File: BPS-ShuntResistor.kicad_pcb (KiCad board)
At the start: 2 copper layers, 37.6 x 32.5 mm, 9 parts, among them J1 Amp_Conn, J2 Conn_01x01_Female, J3 Conn_01x01_Female

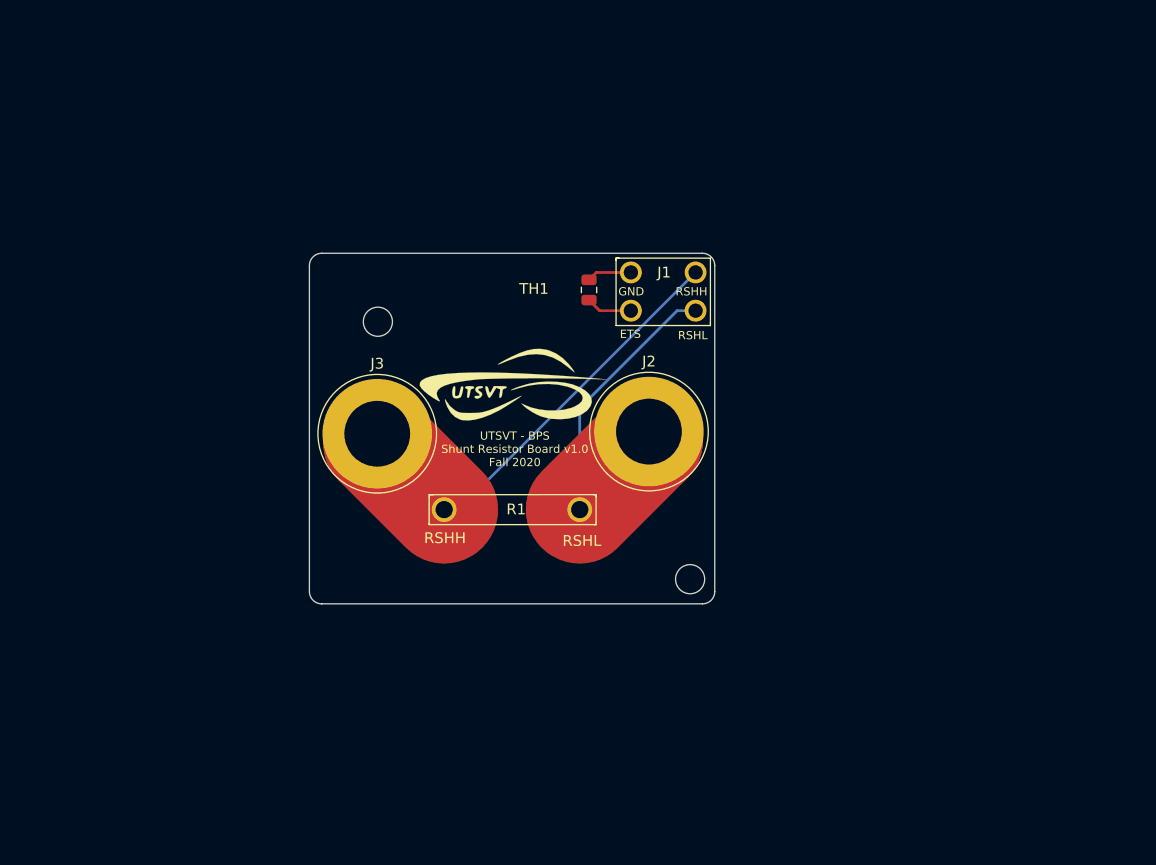
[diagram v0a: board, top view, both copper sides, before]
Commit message: a
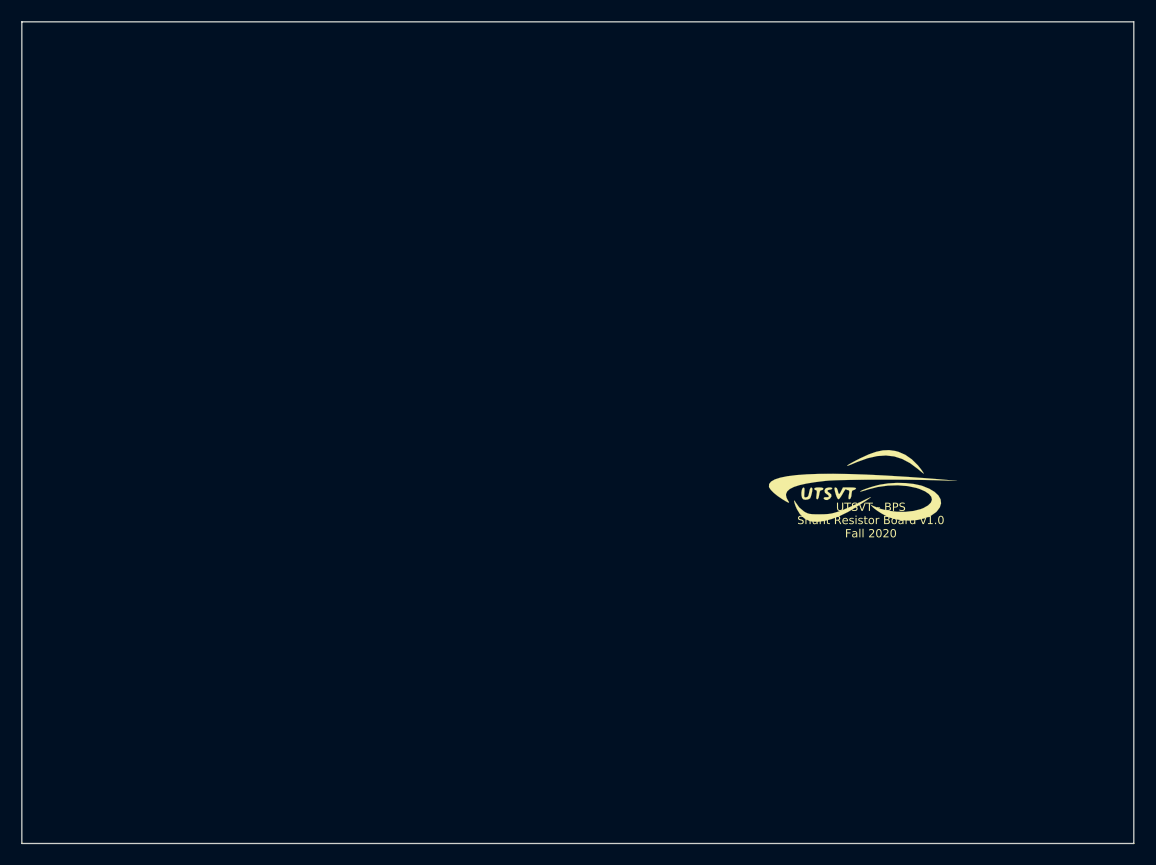
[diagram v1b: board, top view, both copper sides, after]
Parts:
- removed H1, H2: MountingHole, MountingHole:MountingHole_2.7mm_M2.5
- removed J1: Amp_Conn, UTSVT_Connectors:Power_Metal_Strip_Battery_Shunt_Resistor_4_Pin_Connector
- removed J2, J3: Conn_01x01_Female, Connector:Banana_Jack_1Pin
- removed R1: 100u, UTSVT_Passive:Power_Metal_Strip_Battery_Shunt_Resistor
- removed TH1: 100, Resistor_SMD:R_0805_2012Metric
- moved LOGO1 33.7 mm to (194.6, 94.0)
- moved LOGO2 33.7 mm to (195.7, 94.1)
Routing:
- net /RSHH: track 42.3 -> 0.00 mm
- net /RSHL: track 33.8 -> 0.00 mm
- net /ETS: track 4.29 -> 0.00 mm
- net /GND: track 4.17 -> 0.00 mm
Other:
- board size 37.6 x 32.5 mm -> 103.1 x 76.2 mm
- board text removed: "ETS"
- board text removed: "GND"
- board text removed: "RSHH"
- board text removed: "RSHL"
